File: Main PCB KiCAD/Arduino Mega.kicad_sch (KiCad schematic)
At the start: 1 part

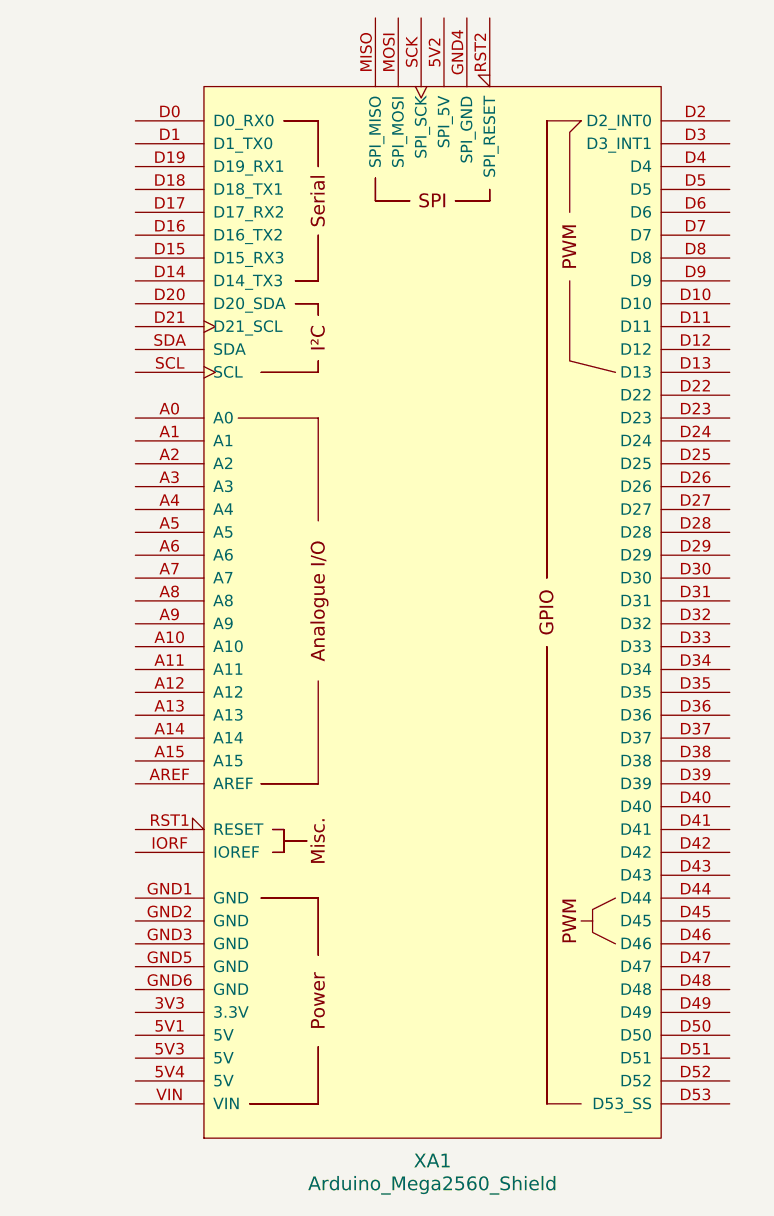
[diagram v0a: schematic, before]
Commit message: cleanup
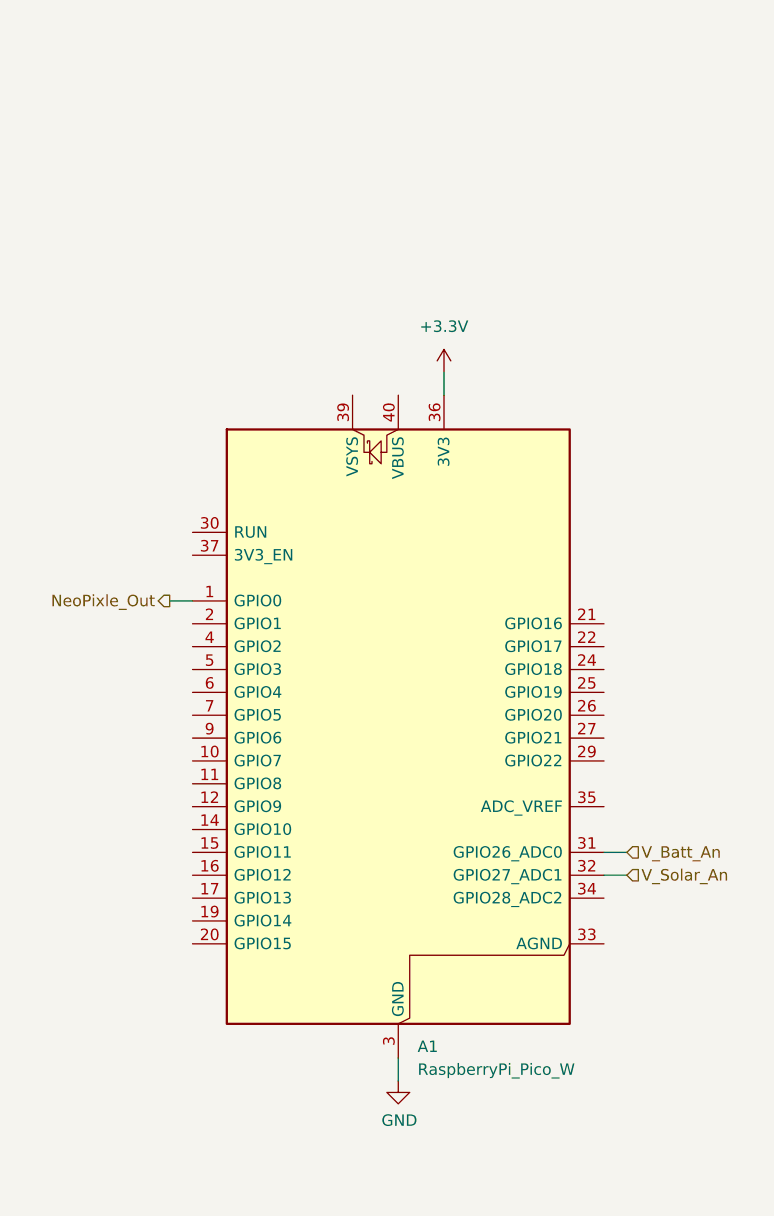
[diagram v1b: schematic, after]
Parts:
- removed XA1: Arduino_Mega2560_Shield, Arduino:Arduino_Mega2560_Shield, symbol Arduino:Arduino_Mega2560_Shield
- added A1: RaspberryPi_Pico_W, Module:RaspberryPi_Pico_Common_Unspecified, symbol MCU_Module:RaspberryPi_Pico_W
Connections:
- new net +3.3V: A1.36 (3V3)
- new net GND: A1.13 (GND), A1.18 (GND), A1.23 (GND), A1.28 (GND), A1.3 (GND), A1.38 (GND), A1.8 (GND)
- new net NeoPixle_Out: A1.1 (GPIO0)
- new net V_Batt_An: A1.31 (GPIO26_ADC0)
- new net V_Solar_An: A1.32 (GPIO27_ADC1)
